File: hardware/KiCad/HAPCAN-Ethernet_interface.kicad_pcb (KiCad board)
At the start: 2 copper layers, 86.5 x 33 mm, 55 parts, among them CON1 Connectors CAN bus, IC1 MCP16301HT, IC2 FT230XS, IC3 USBLC6-2SC6, IC4 MCP2561-E-SN, IC5 STM32F072C8Tx, U1 HLK-7628N

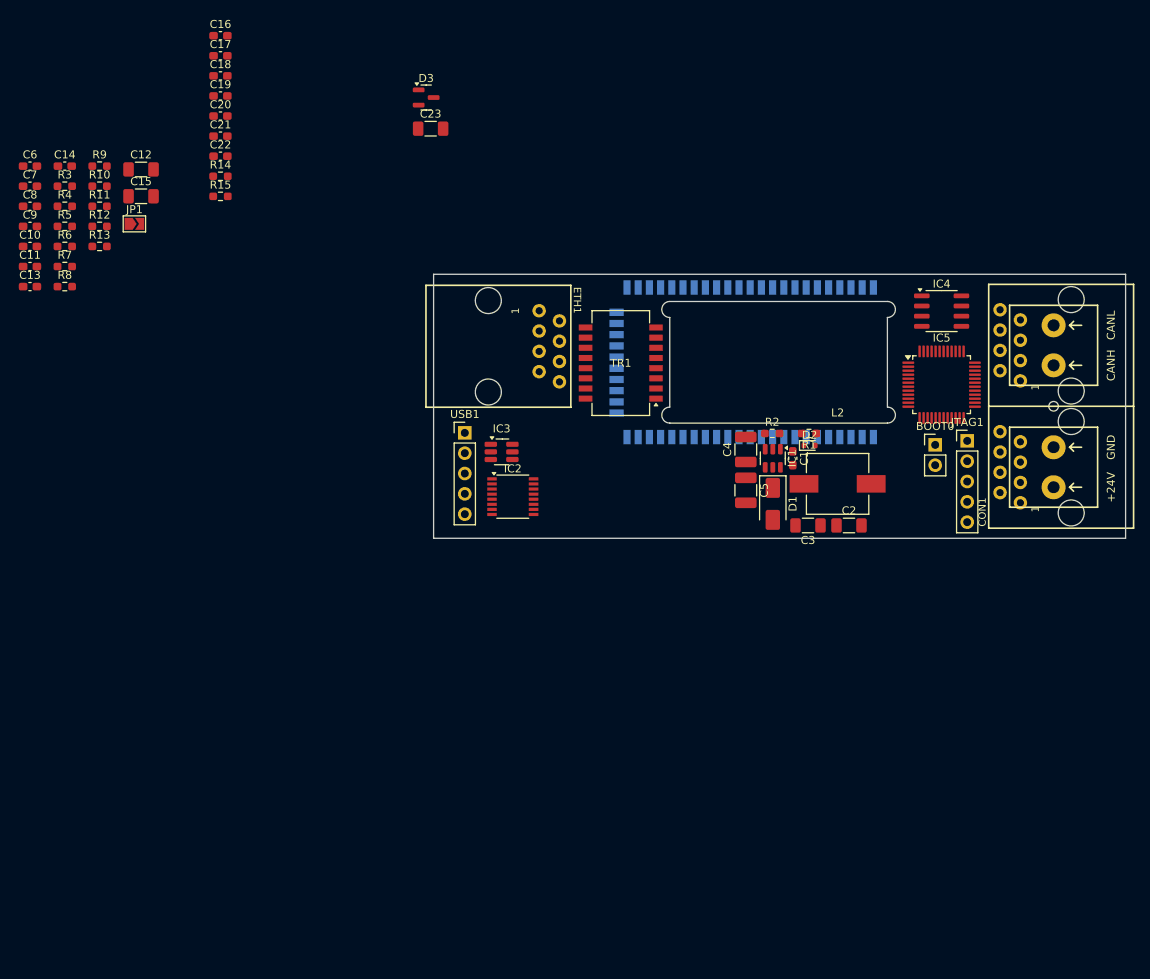
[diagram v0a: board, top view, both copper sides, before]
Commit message: Finished schematic, but needs cleanup. Started component placement on board.
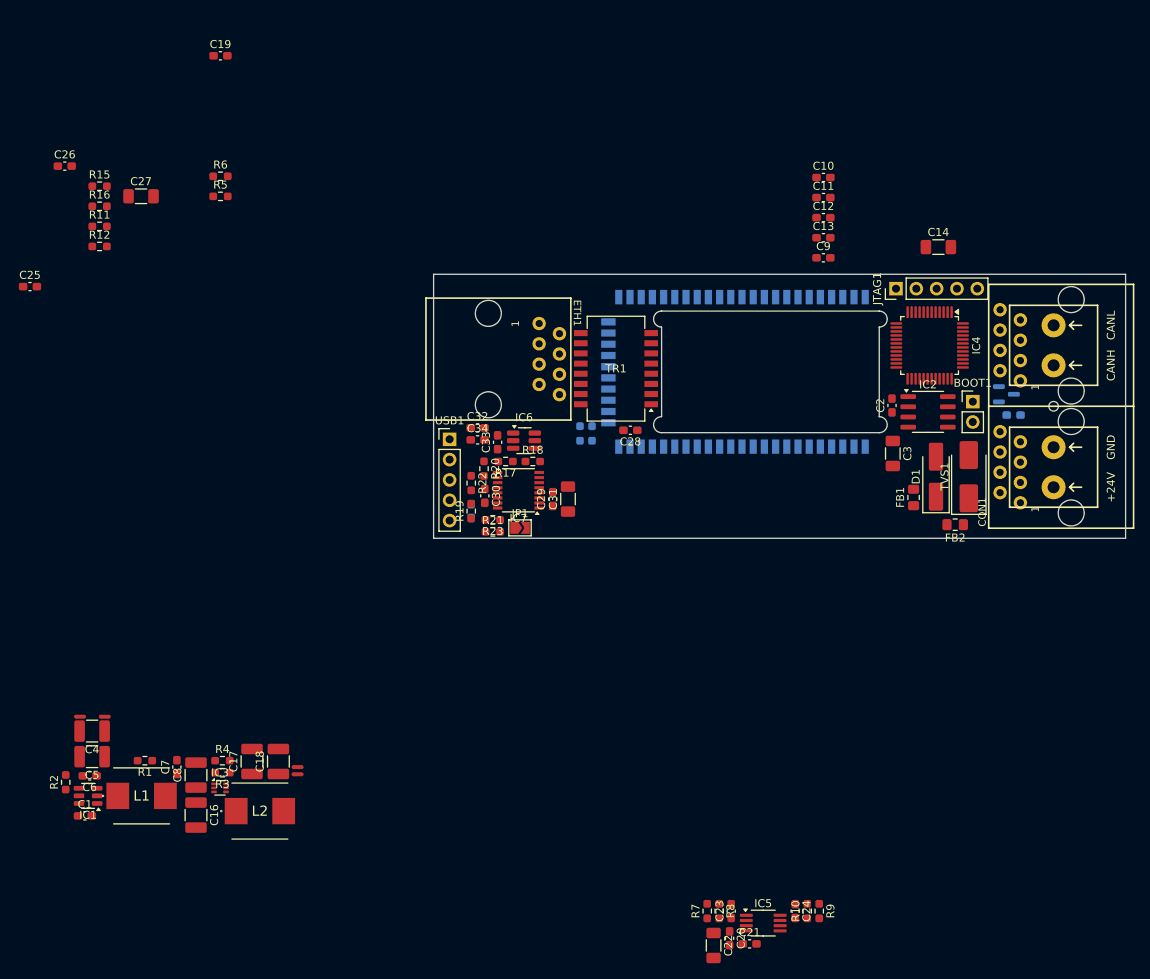
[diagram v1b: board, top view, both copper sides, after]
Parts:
- removed D2: BAS521-QX, Diode_SMD:D_SOD-523
- added C15: 100n, Capacitor_SMD:C_0603_1608Metric_Pad1.08x0.95mm_HandSolder, B.Cu at (172.5, 117.6)
- added C16: 10u 16V, Capacitor_SMD:C_1210_3225Metric_Pad1.33x2.70mm_HandSolder, F.Cu at (70.3, 167.6)
- added C17: 10u 10V, Capacitor_SMD:C_1210_3225Metric_Pad1.33x2.70mm_HandSolder, F.Cu at (77.3, 160.9)
- added C18: 22u 10V, Capacitor_SMD:C_1210_3225Metric_Pad1.33x2.70mm_HandSolder, F.Cu at (80.6, 160.9)
- added C20: 10n, Capacitor_SMD:C_0603_1608Metric_Pad1.08x0.95mm_HandSolder, F.Cu at (137.0, 183.0)
- added C21: 100n, Capacitor_SMD:C_0603_1608Metric_Pad1.08x0.95mm_HandSolder, F.Cu at (139.5, 183.7)
- added C22: 10u 6.3V, Capacitor_SMD:C_1206_3216Metric_Pad1.33x1.80mm_HandSolder, F.Cu at (135.0, 183.9)
- added C23: 100n, Capacitor_SMD:C_0603_1608Metric_Pad1.08x0.95mm_HandSolder, F.Cu at (137.2, 179.6)
- added C24: 100n, Capacitor_SMD:C_0603_1608Metric_Pad1.08x0.95mm_HandSolder, F.Cu at (145.2, 179.6)
- added C6: 100n, Capacitor_SMD:C_0603_1608Metric_Pad1.08x0.95mm_HandSolder, F.Cu at (57.0, 162.7)
- added C7: 100n, Capacitor_SMD:C_0603_1608Metric_Pad1.08x0.95mm_HandSolder, F.Cu at (67.9, 161.6)
- added C8: 10u 16V, Capacitor_SMD:C_1210_3225Metric_Pad1.33x2.70mm_HandSolder, F.Cu at (70.3, 162.6)
- added FB1: 1k@100MHz, Inductor_SMD:L_0805_2012Metric_Pad1.15x1.40mm_HandSolder, F.Cu at (160.0, 127.9)
- added FB2: 1k@100MHz, Inductor_SMD:L_0805_2012Metric_Pad1.15x1.40mm_HandSolder, F.Cu at (165.2, 131.3)
- added IC3: TLV62568DRL, Package_TO_SOT_SMD:SOT-563, F.Cu at (73.3, 164.2)
- added IC5: MCP3422A0-E/MS, Package_SO:MSOP-8_3x3mm_P0.65mm, F.Cu at (141.2, 181.1)
- added L1: 3.3uH, ProjectLib:SPM7054VT, F.Cu at (63.5, 165.2)
- added NT1: NetTie_2, NetTie:NetTie-2_SMD_Pad0.5mm, F.Cu at (58.9, 155.3)
- added NT2: NetTie_2, NetTie:NetTie-2_SMD_Pad0.5mm, F.Cu at (55.8, 155.3)
- added NT3: NetTie_2, NetTie:NetTie-2_SMD_Pad0.5mm, F.Cu at (83.0, 162.5)
- added NT4: NetTie_2, NetTie:NetTie-2_SMD_Pad0.5mm, F.Cu at (83.0, 161.6)
- added R10: 22k, Resistor_SMD:R_0603_1608Metric_Pad0.98x0.95mm_HandSolder, F.Cu at (146.7, 179.6)
- added R13: 10k, Resistor_SMD:R_0603_1608Metric_Pad0.98x0.95mm_HandSolder, B.Cu at (119.8, 119.9)
- added R14: 10k, Resistor_SMD:R_0603_1608Metric_Pad0.98x0.95mm_HandSolder, B.Cu at (118.3, 119.9)
- added R3: 100k, Resistor_SMD:R_0603_1608Metric_Pad0.98x0.95mm_HandSolder, F.Cu at (73.6, 162.3)
- added R4: 22k, Resistor_SMD:R_0603_1608Metric_Pad0.98x0.95mm_HandSolder, F.Cu at (73.6, 160.8)
- added R7: 330k, Resistor_SMD:R_0603_1608Metric_Pad0.98x0.95mm_HandSolder, F.Cu at (134.2, 179.6)
- added R8: 22k, Resistor_SMD:R_0603_1608Metric_Pad0.98x0.95mm_HandSolder, F.Cu at (135.7, 179.6)
- added R9: 22k, Resistor_SMD:R_0603_1608Metric_Pad0.98x0.95mm_HandSolder, F.Cu at (148.2, 179.6)
- added TVS1: P6SMB33CA, Diode_SMD:D_SMB_Handsoldering, F.Cu at (166.9, 125.3)
- C2: value 10u 6.3V -> 100n; footprint Capacitor_SMD:C_1206_3216Metric_Pad1.33x1.80mm_HandSolder -> Capacitor_SMD:C_0603_1608Metric_Pad1.08x0.95mm_HandSolder
- C3: value 10u 6.3V -> 10u 10V
- C35: renamed from C6; moved to B.Cu
- D1: value B140Q -> US1D; footprint Diode_SMD:D_SMA -> Diode_SMD:D_SMA_Handsoldering
- IC1: value MCP16301HT -> LMR51430Y
- L2: value 15uH -> 1uH; footprint Inductor_SMD:L_Wuerth_WE-PD-Typ-M-Typ-S_Handsoldering -> ProjectLib:SPM7054VT
- R1: value 31k6 -> 200k
- R2: value 10k -> 27k
- TVS2: renamed from D3; moved to B.Cu
- moved C1 99.1 mm to (56.4, 167.7), turned to 0 degrees
- moved R2 98.5 mm to (54.0, 163.5), turned to 90 degrees
- moved IC1 95.4 mm to (56.8, 165.2), turned to 180 degrees
- moved R1 92.5 mm to (63.9, 160.8)
- moved C4 89.0 mm to (57.3, 157.1), turned to 180 degrees
- moved C5 88.2 mm to (57.3, 160.3), turned to 180 degrees
- moved L2 83.0 mm to (78.3, 167.1)
- moved TVS2 81.5 mm to (171.6, 115.0)
- moved C10 76.4 mm to (148.7, 87.9)
- moved C11 76.4 mm to (148.7, 90.4)
- moved C12 76.4 mm to (148.7, 92.9)
- moved C13 76.4 mm to (148.7, 95.4)
- moved C9 76.4 mm to (148.7, 97.9)
- moved C29 73.7 mm to (114.9, 128.1), turned to 90 degrees
- moved C28 71.1 mm to (124.6, 119.5), turned to 180 degrees
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- renumbered BOOT0 to BOOT1, C18 to C10, C19 to C11, C20 to C12, C21 to C13, C23 to C14, C17 to C19, C13 to C25, C14 to C26, C15 to C27, C16 to C28, C9 to C29, C11 to C30, C12 to C31, C10 to C32, C7 to C33, C8 to C34, C22 to C9, IC4 to IC2, IC5 to IC4, IC3 to IC6, IC2 to IC7, R12 to R11, R13 to R12, R10 to R15, R11 to R16, R8 to R17, R9 to R18, R3 to R19, R4 to R20, R6 to R21, R5 to R22, R7 to R23, R15 to R5, R14 to R6
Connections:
- C1 pad 1: Net-(D2-K) -> Net-(IC1-CB)
- C1 pad 2: Net-(D1-K) -> Net-(IC1-SW)
- C2 pad 1: +3V3 -> +5V
- C3 pad 1: +3V3 -> +5V
- CON1 pad +24V: unconnected-(CON1-Pad+24V) -> Net-(D1-A)
- CON1 pad CANH: unconnected-(CON1-PadCANH) -> /CANH
- CON1 pad CANL: unconnected-(CON1-PadCANL) -> /CANL
- CON1 pad GND: unconnected-(CON1-PadGND) -> GNDPWR
- D1 pad 2: GND -> Net-(D1-A)
- IC1 pad 1: Net-(D2-K) -> GND
- IC1 pad 2: GND -> Net-(IC1-SW)
- IC1 pad 3: Net-(IC1-Vfb) -> +24V
- IC1 pad 4: +24V -> Net-(IC1-FB)
- IC1 pad 6: Net-(D1-K) -> Net-(IC1-CB)
- IC2 pad 1: unconnected-(IC4-TXD-Pad1) -> /CAN_Tx
- IC2 pad 2: unconnected-(IC4-VSS-Pad2) -> GND
- IC2 pad 3: unconnected-(IC4-VDD-Pad3) -> +5V
- IC2 pad 4: unconnected-(IC4-RXD-Pad4) -> /CAN_Rx
- IC2 pad 6: unconnected-(IC4-CANL-Pad6) -> /CANL
- IC2 pad 7: unconnected-(IC4-CANH-Pad7) -> /CANH
- IC2 pad 8: unconnected-(IC4-STBY-Pad8) -> GND
- IC4 pad 32: unconnected-(IC5-PA11-Pad32) -> /CAN_USB_D-
- IC4 pad 33: unconnected-(IC5-PA12-Pad33) -> /CAN_USB_D+
- IC4 pad 34: unconnected-(IC5-PA13-Pad34) -> /SWDIO
- IC4 pad 37: unconnected-(IC5-PA14-Pad37) -> /SWCLK
- IC4 pad 45: unconnected-(IC5-PB8-Pad45) -> /CAN_Rx
- IC4 pad 46: unconnected-(IC5-PB9-Pad46) -> /CAN_Tx
- IC6 pad 1: Net-(USB1-D+) -> Net-(USB1-D-)
- IC6 pad 3: Net-(USB1-D-) -> Net-(USB1-D+)
- L2 pad 1: Net-(D1-K) -> Net-(IC3-SW)
- R1 pad 1: +3V3 -> +5V
- R1 pad 2: Net-(IC1-Vfb) -> Net-(IC1-FB)
- R17 pad 2: /D+ -> /D-
- R18 pad 2: /D- -> /D+
- R2 pad 1: Net-(IC1-Vfb) -> Net-(IC1-FB)
- TVS2 pad 1: unconnected-(D3-K-Pad1) -> /CANH
- TVS2 pad 2: unconnected-(D3-K-Pad2) -> /CANL
- TVS2 pad 3: unconnected-(D3-A-Pad3) -> GNDPWR
- U1 pad 24: unconnected-(U1-I2C_SCLK-Pad24) -> /I2C_CLK
- U1 pad 25: unconnected-(U1-I2C_SD-Pad25) -> /I2C_SDA
- U1 pad 54: unconnected-(U1-USB_DP-Pad54) -> /CAN_USB_D+
- U1 pad 55: unconnected-(U1-USB_DM-Pad55) -> /CAN_USB_D-
